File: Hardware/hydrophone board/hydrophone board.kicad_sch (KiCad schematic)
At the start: 0 parts

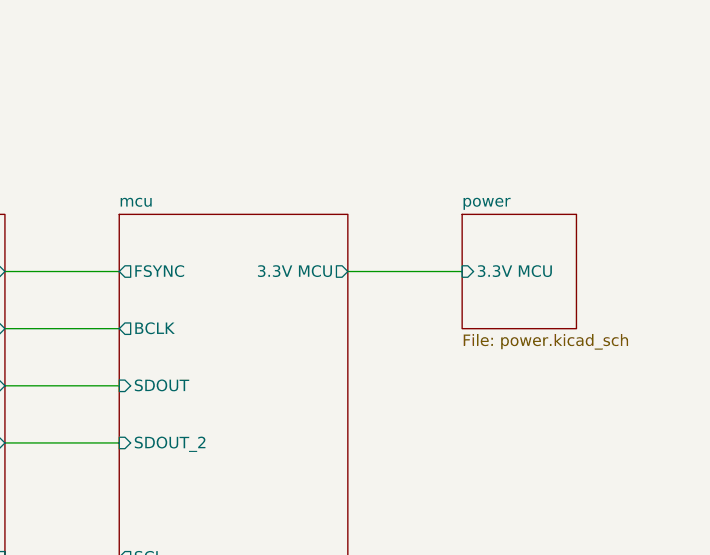
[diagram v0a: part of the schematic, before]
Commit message: Revert "Merge branch 'hardware' of https://github.com/bruin-underwater-robotics/2023-2024 into hardware"
This reverts commit 1d5f0f31a35e539c7b0b2eac7ff2db3bf82506a7, reversing
changes made to b9b3862216192341382b87943b4a1d0c2c46b631.
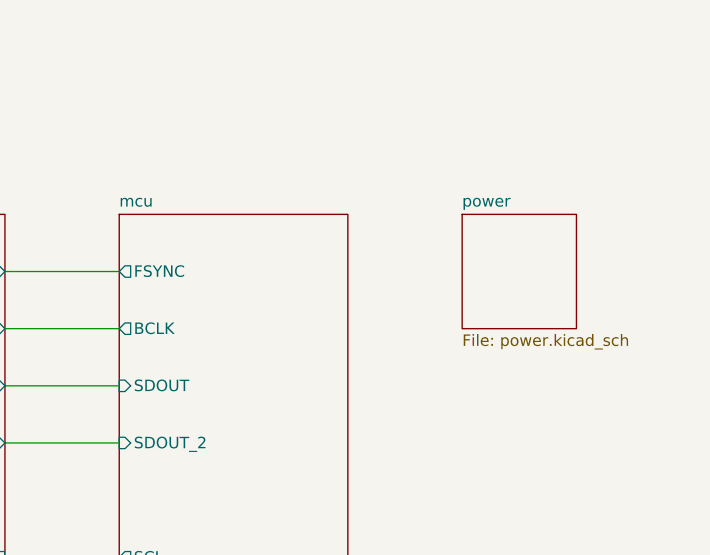
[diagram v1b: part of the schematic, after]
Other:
- sheet mcu ports: added none; removed 3.3V MCU
- sheet power ports: added none; removed 3.3V MCU
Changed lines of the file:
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@@
-    (stroke (width 0) (type default))
-  )
-  (wire (pts (xy 228.6 76.2) (xy 241.3 76.2))
     (stroke (width 0) (type default))
   )
@@
     (pin "BCLK" output (at 203.2 82.55 180)
       (effects (font (size 1.27 1.27)) (justify left))
-    )
-    (pin "3.3V MCU" output (at 228.6 76.2 0)
-      (effects (font (size 1.27 1.27)) (justify right))
     )
     (instances
@@
       (effects (font (size 1.27 1.27)) (justify left top))
     )
-    (pin "3.3V MCU" input (at 241.3 76.2 180)
-      (effects (font (size 1.27 1.27)) (justify left))
-    )
     (instances

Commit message: 3.3v connector
on power sheet
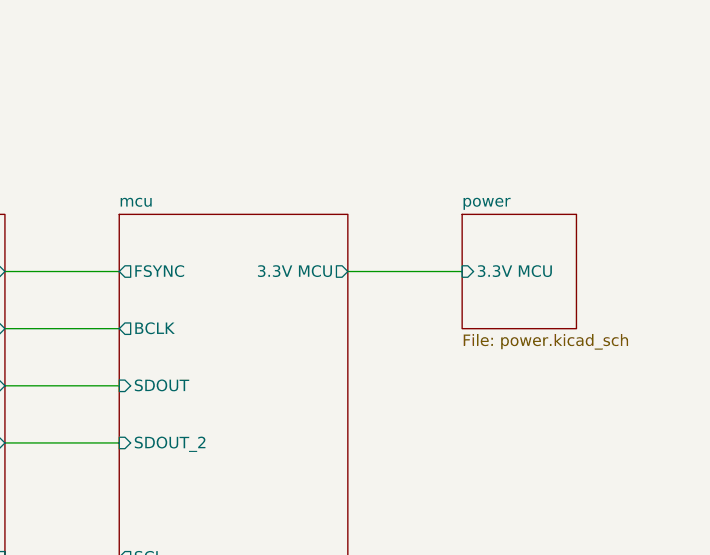
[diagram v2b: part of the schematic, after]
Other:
- sheet mcu ports: added 3.3V MCU; removed none
- sheet power ports: added 3.3V MCU; removed none
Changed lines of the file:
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@@
+    (stroke (width 0) (type default))
+  )
+  (wire (pts (xy 228.6 76.2) (xy 241.3 76.2))
     (stroke (width 0) (type default))
   )
@@
       (effects (font (size 1.27 1.27)) (justify left))
     )
+    (pin "3.3V MCU" output (at 228.6 76.2 0)
+      (effects (font (size 1.27 1.27)) (justify right))
+    )
     (instances
       (project "hydrophone board"
@@
       (effects (font (size 1.27 1.27)) (justify left top))
     )
-    (instances
+    (pin "3.3V MCU" input (at 241.3 76.2 180)
+      (effects (font (size 1.27 1.27)) (justify left))
+    )
+    (instances
